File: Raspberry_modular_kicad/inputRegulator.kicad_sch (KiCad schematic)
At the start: 4 parts

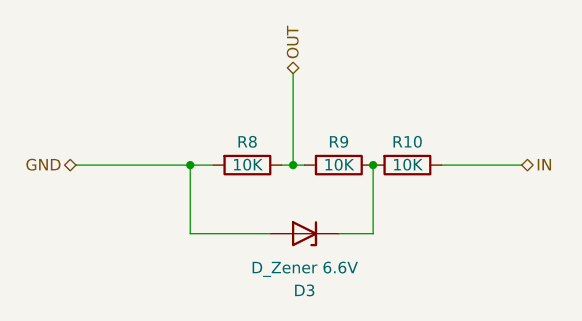
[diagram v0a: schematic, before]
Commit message: [UDPT] Electricals footprints
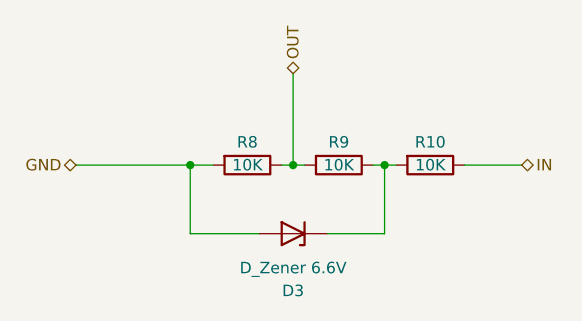
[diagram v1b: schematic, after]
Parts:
- D3: footprint Raspberry_modular:D_0603_1608Metric -> Modular Shield:D_0603_1608Metric
- R10, R8, R9: footprint Raspberry_modular:R_0603_1608Metric -> Modular Shield:R_0603_1608Metric
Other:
- moved on the sheet: D3, R10
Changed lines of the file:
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@@
   (junction (at 33.02 30.48) (diameter 0) (color 0 0 0 0)
   )
-  (junction (at 53.34 30.48) (diameter 0) (color 0 0 0 0)
+  (junction (at 54.61 30.48) (diameter 0) (color 0 0 0 0)
   )
   (junction (at 44.45 30.48) (diameter 0) (color 0 0 0 0)
@@
     (stroke (width 0) (type default))
   )
-  (wire (pts (xy 53.34 38.1) (xy 53.34 30.48))
+  (wire (pts (xy 54.61 38.1) (xy 54.61 30.48))
+    (stroke (width 0) (type default))
+  )
+  (wire (pts (xy 54.61 30.48) (xy 53.34 30.48))
     (stroke (width 0) (type default))
   )
@@
     (stroke (width 0) (type default))
   )
+  (wire (pts (xy 55.88 30.48) (xy 54.61 30.48))
+    (stroke (width 0) (type default))
+  )
   (wire (pts (xy 20.32 30.48) (xy 33.02 30.48))
     (stroke (width 0) (type default))
   )
-  (wire (pts (xy 41.91 38.1) (xy 33.02 38.1))
+  (wire (pts (xy 40.64 38.1) (xy 33.02 38.1))
     (stroke (width 0) (type default))
   )
@@
     (stroke (width 0) (type default))
   )
-  (wire (pts (xy 49.53 38.1) (xy 53.34 38.1))
-    (stroke (width 0) (type default))
-  )
-  (wire (pts (xy 60.96 30.48) (xy 69.85 30.48))
+  (wire (pts (xy 48.26 38.1) (xy 54.61 38.1))
+    (stroke (width 0) (type default))
+  )
+  (wire (pts (xy 63.5 30.48) (xy 69.85 30.48))
     (stroke (width 0) (type default))
   )
@@
       (effects (font (size 1.27 1.27)))
     )
-    (property "Footprint" "Raspberry_modular:R_0603_1608Metric" (at 49.53 28.702 90)
+    (property "Footprint" "Modular Shield:R_0603_1608Metric" (at 49.53 28.702 90)
       (effects (font (size 1.27 1.27)) hide)
     )
@@
     )
   )
-  (symbol (lib_id "Modular Shield:R") (at 57.15 30.48 270) (unit 1)
-    (in_bom yes) (on_board yes) (dnp no)
-    (property "Reference" "R10" (at 57.15 27.94 90)
-      (effects (font (size 1.27 1.27)))
-    )
-    (property "Value" "10K" (at 57.15 30.48 90)
-      (effects (font (size 1.27 1.27)))
-    )
-    (property "Footprint" "Raspberry_modular:R_0603_1608Metric" (at 57.15 28.702 90)
-      (effects (font (size 1.27 1.27)) hide)
-    )
-    (property "Datasheet" "~" (at 57.15 30.48 0)
+  (symbol (lib_id "Modular Shield:R") (at 59.69 30.48 270) (unit 1)
+    (in_bom yes) (on_board yes) (dnp no)
+    (property "Reference" "R10" (at 59.69 27.94 90)
+      (effects (font (size 1.27 1.27)))
+    )
+    (property "Value" "10K" (at 59.69 30.48 90)
+      (effects (font (size 1.27 1.27)))
+    )
+    (property "Footprint" "Modular Shield:R_0603_1608Metric" (at 59.69 28.702 90)
+      (effects (font (size 1.27 1.27)) hide)
+    )
+    (property "Datasheet" "~" (at 59.69 30.48 0)
       (effects (font (size 1.27 1.27)) hide)
     )
@@
       (effects (font (size 1.27 1.27)))
     )
-    (property "Footprint" "Raspberry_modular:R_0603_1608Metric" (at 39.37 28.702 90)
+    (property "Footprint" "Modular Shield:R_0603_1608Metric" (at 39.37 28.702 90)
       (effects (font (size 1.27 1.27)) hide)
     )
@@
     )
   )
-  (symbol (lib_id "Modular Shield:D_Zener") (at 45.72 38.1 180) (unit 1)
-    (in_bom yes) (on_board yes) (dnp no)
-    (property "Reference" "D3" (at 45.72 44.45 0)
-      (effects (font (size 1.27 1.27)))
-    )
-    (property "Value" "D_Zener 6.6V" (at 45.72 41.91 0)
-      (effects (font (size 1.27 1.27)))
-    )
-    (property "Footprint" "Raspberry_modular:D_0603_1608Metric" (at 45.72 38.1 0)
-      (effects (font (size 1.27 1.27)) hide)
-    )
-    (property "Datasheet" "~" (at 45.72 38.1 0)
-      (effects (font (size 1.27 1.27)) hide)
-    )
+  (symbol (lib_id "Modular Shield:D_Zener") (at 44.45 38.1 180) (unit 1)
+    (in_bom yes) (on_board yes) (dnp no)
+    (property "Reference" "D3" (at 44.45 44.45 0)
+      (effects (font (size 1.27 1.27)))
+    )
+    (property "Value" "D_Zener 6.6V" (at 44.45 41.91 0)
+      (effects (font (size 1.27 1.27)))
+    )
+    (property "Footprint" "Modular Shield:D_0603_1608Metric" (at 44.45 38.1 0)
+      (effects (font (size 1.27 1.27)) hide)
+    )
+    (property "Datasheet" "~" (at 44.45 38.1 0)
+      (effects (font (size 1.27 1.27)) hide)
+    )

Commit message: [ADD] Bom
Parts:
- D3: LCSC (none) -> C894569
- R10, R8, R9: LCSC (none) -> C25804
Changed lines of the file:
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@@
+      (effects (font (size 1.27 1.27)) hide)
+    )
+    (property "LCSC" "C25804" (at 49.53 34.29 90)
       (effects (font (size 1.27 1.27)) hide)
     )
@@
       (effects (font (size 1.27 1.27)) hide)
     )
+    (property "LCSC" "C25804" (at 59.69 34.29 90)
+      (effects (font (size 1.27 1.27)) hide)
+    )
     (pin "1")
     (pin "2")
@@
       (effects (font (size 1.27 1.27)) hide)
     )
+    (property "LCSC" "C25804" (at 39.37 34.29 90)
+      (effects (font (size 1.27 1.27)) hide)
+    )
     (pin "1")
     (pin "2")
@@
       (effects (font (size 1.27 1.27)) hide)
     )
+    (property "LCSC" "C894569" (at 44.45 44.45 0)
+      (effects (font (size 1.27 1.27)) hide)
+    )
